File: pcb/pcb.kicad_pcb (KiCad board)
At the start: 2 copper layers, 80 parts, among them J1 USB_B_Micro, J2 battery, J3 SD_Card, J4 swd, J5 speakers, SW1 RotaryEncoder, SW2 next, SW3 play, U1 TP4056, U2 LM358, U3 ME2149, U4 PCM1754, U5 CC2640, U6 LM4810, U7 LM358, Y1 24M

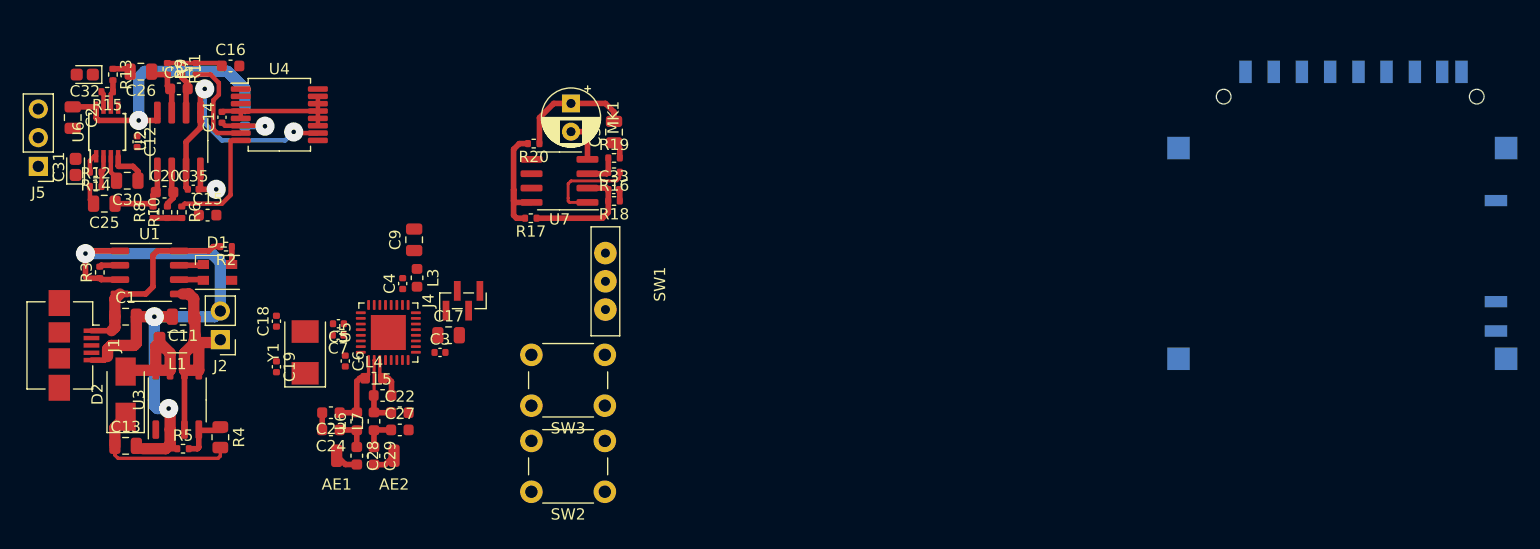
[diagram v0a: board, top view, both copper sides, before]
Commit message: 4.5x4 pcb
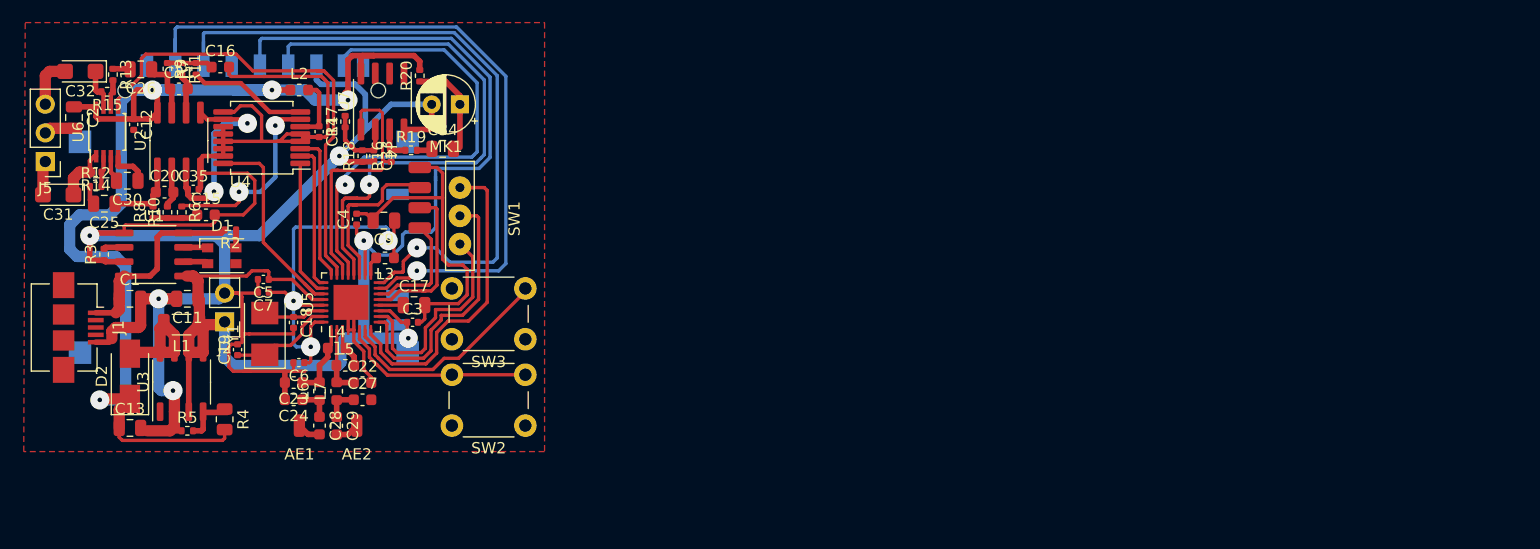
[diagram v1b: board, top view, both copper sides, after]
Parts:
- C31, C32: footprint Capacitor_Tantalum_SMD:CP_EIA-1608-08_AVX-J -> Capacitor_Tantalum_SMD:CP_EIA-3216-10_Kemet-I
- J4: footprint Connector_PinHeader_1.00mm:PinHeader_1x04_P1.00mm_Vertical_SMD_Pin1Left -> local:swd
- L2: moved to F.Cu
- moved J3 97.2 mm to (124.5, 67.1)
- moved R18 22.6 mm to (135.0, 60.2), turned to 90 degrees
- moved C33 21.4 mm to (136.0, 60.2), turned to -90 degrees
- moved R16 19.8 mm to (137.5, 60.2), turned to 90 degrees
- moved R17 18.5 mm to (133.5, 57.1), turned to 90 degrees
- moved R19 18.0 mm to (139.3, 59.7)
- moved U7 17.2 mm to (136.8, 55.4), turned to 90 degrees
- moved C34 15.2 mm to (142.1, 59.6), turned to 0 degrees
- moved SW1 14.1 mm to (143.6, 65.5)
- moved R20 11.7 mm to (140.1, 53.1), turned to 90 degrees
- moved J4 9.90 mm to (140.1, 63.9), turned to -90 degrees
- moved MK1 9.83 mm to (143.6, 55.6), turned to 180 degrees
- moved SW3 9.17 mm to (149.4, 76.4)
- moved SW2 9.16 mm to (149.4, 84.1)
- moved C14 8.70 mm to (131.2, 58.0), turned to -90 degrees
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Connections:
- J3 pad 2: Net-(J3-Pad2) -> Net-(U5-Pad16)
- J3 pad 5: Net-(J3-Pad5) -> Net-(U5-Pad20)
- U4 pad 7: Net-(R7-Pad1) -> Net-(R6-Pad1)
- U4 pad 8: Net-(R6-Pad1) -> Net-(R7-Pad1)
- U5 pad 15: Net-(J3-Pad7) -> Net-(J3-Pad1)
- U5 pad 16: Net-(J3-Pad5) -> Net-(U5-Pad16)
- U5 pad 20: Net-(J3-Pad2) -> Net-(U5-Pad20)
- U5 pad 21: Net-(J3-Pad1) -> Net-(J3-Pad7)
- U5 pad 24: /ADC_SCK -> /ADC_LRCLK
- U5 pad 25: /ADC_BCK -> /ADC_DATA
- U5 pad 26: /ADC_DATA -> /ADC_BCK
- U5 pad 27: /ADC_LRCLK -> /ADC_SCK
- U5 pad 4: unconnected-(U5-Pad4) -> GND
- U5 pad 5: unconnected-(U5-Pad5) -> GND
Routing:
- net GND: track 83.2 -> 236.7 mm
- net +4V: track 19.6 -> 123.8 mm, vias 0 -> 2
- net Net-(J3-Pad1): track 0.00 -> 65.5 mm, vias 0 -> 1
- net Net-(U5-Pad16): track 0.00 -> 61.7 mm, vias 0 -> 1
- net +6V: track 52.3 -> 113.7 mm, vias 1 -> 4
- net Net-(U5-Pad20): track 0.00 -> 50.9 mm, vias 0 -> 1
- net /PA_SDN: track 0.00 -> 43.1 mm
- net Net-(J3-Pad7): track 0.00 -> 42.2 mm, vias 0 -> 1
- net +VSW: track 0.00 -> 35.0 mm, vias 0 -> 3
- net Net-(SW1-PadB): track 0.00 -> 29.9 mm
- net Net-(SW1-PadC): track 0.00 -> 25.6 mm
- net Net-(SW1-PadA): track 0.00 -> 19.7 mm
- net Net-(SW3-Pad2): track 0.00 -> 19.5 mm
- net /ADC_SCK: track 0.00 -> 18.6 mm
- net Net-(SW2-Pad2): track 0.00 -> 17.3 mm
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- added copper zone on F.Cu, net GND
